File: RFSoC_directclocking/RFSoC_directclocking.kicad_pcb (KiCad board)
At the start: 2 copper layers, 54.6 x 43.2 mm, 16 parts, among them U1 TCM2-33WX+, U2 TCM2-33WX+

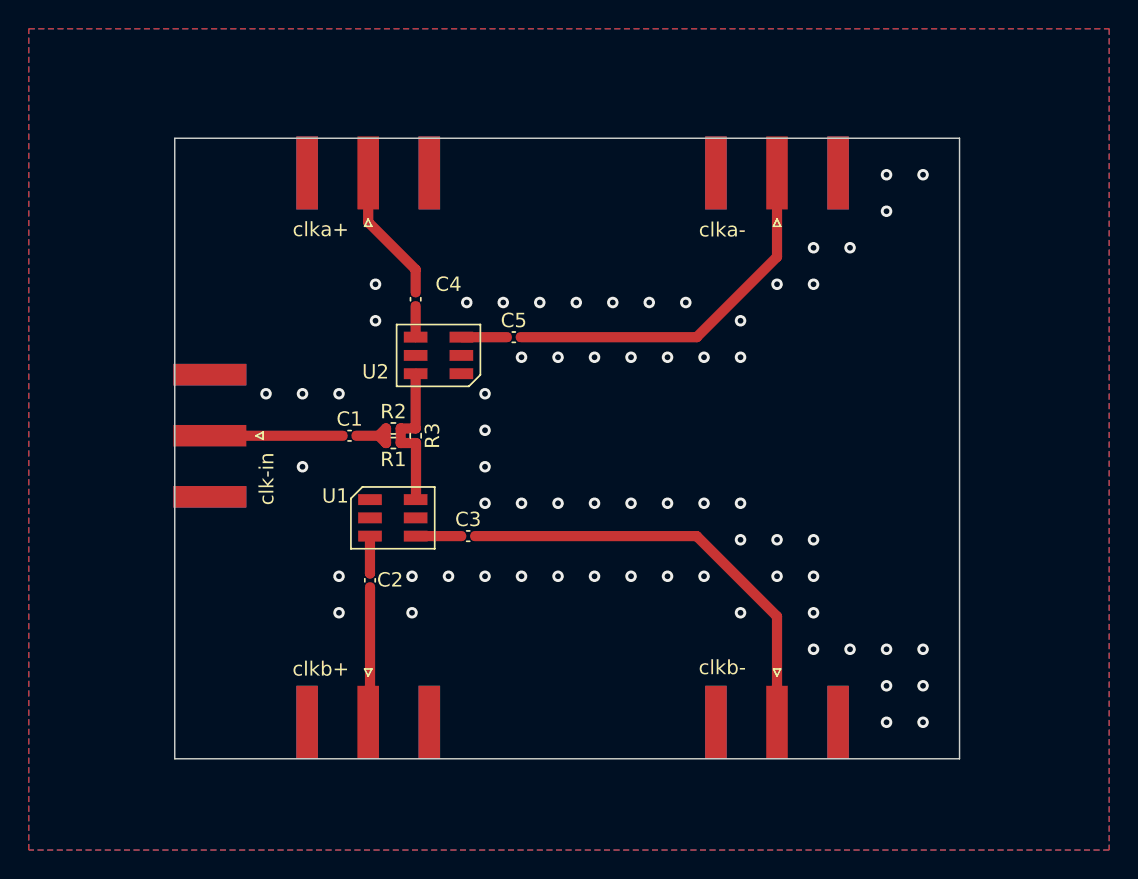
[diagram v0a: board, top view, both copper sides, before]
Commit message: mc lib components
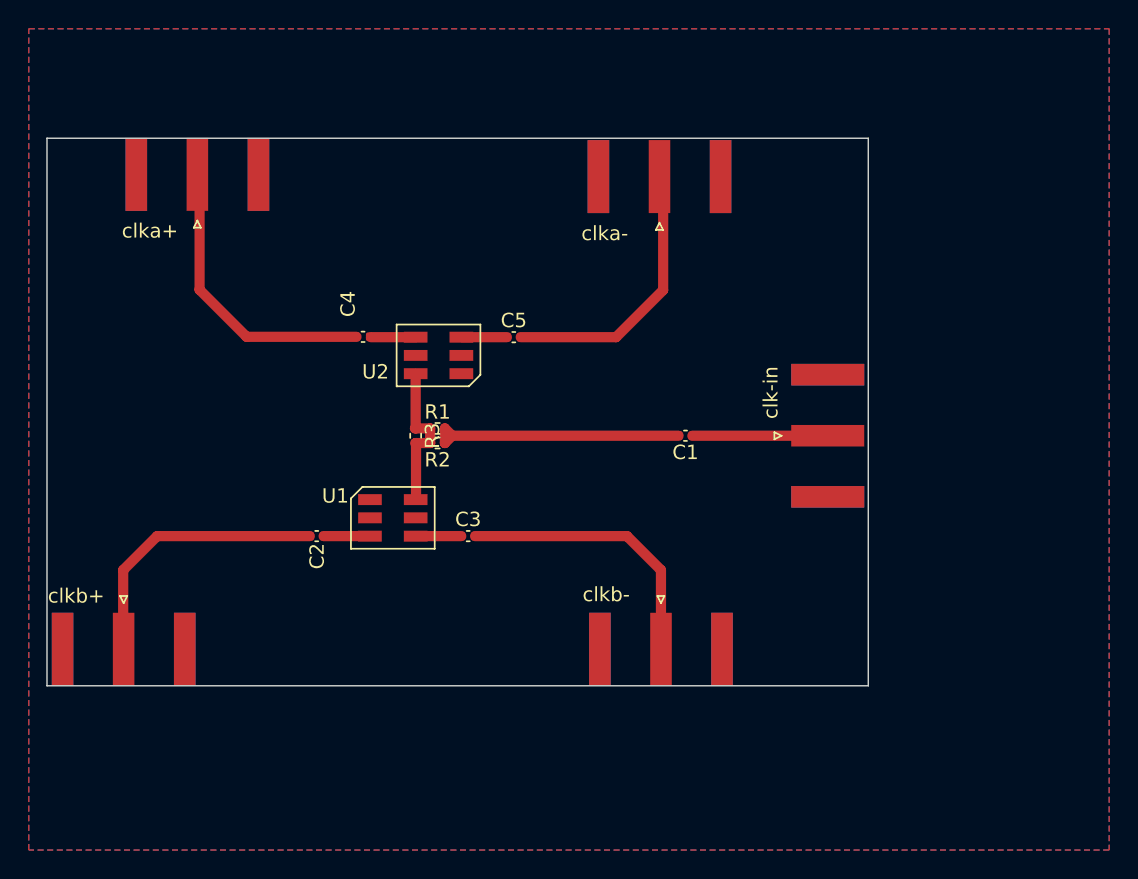
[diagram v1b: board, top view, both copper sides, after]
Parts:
- moved clk-in 43.0 mm to (128.0, 79.1), turned to 0 degrees
- moved C1 23.4 mm to (118.1, 79.1), turned to 180 degrees
- moved clkb+ 17.8 mm to (79.0, 94.0)
- moved clka+ 11.9 mm to (84.1, 60.9)
- moved clkb- 9.54 mm to (116.4, 94.0)
- moved clka- 8.18 mm to (116.3, 61.1)
- moved C2 4.82 mm to (92.4, 86.1), turned to 180 degrees
- moved C4 4.50 mm to (95.7, 72.2), turned to 180 degrees
- moved R1 3.24 mm to (100.8, 78.6), turned to 180 degrees
- moved R2 3.24 mm to (100.8, 79.6), turned to 180 degrees
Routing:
- net Net-(C1-Pad2): track 4.00 -> 18.2 mm
- net Net-(C3-Pad2): track 30.4 -> 19.4 mm
- net Net-(C2-Pad2): track 9.14 -> 19.5 mm
- net Net-(C4-Pad2): track 9.68 -> 18.9 mm
- net Net-(C5-Pad2): track 26.0 -> 18.9 mm
- net Net-(C4-Pad1): track 2.16 -> 3.17 mm
- net Net-(C2-Pad1): track 2.60 -> 3.23 mm
- net GND: vias 66 -> 0
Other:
- board size 54.6 x 43.2 mm -> 57.2 x 38.1 mm
